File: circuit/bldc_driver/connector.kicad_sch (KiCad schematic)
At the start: 13 parts, among them J4 PH2.0_6P

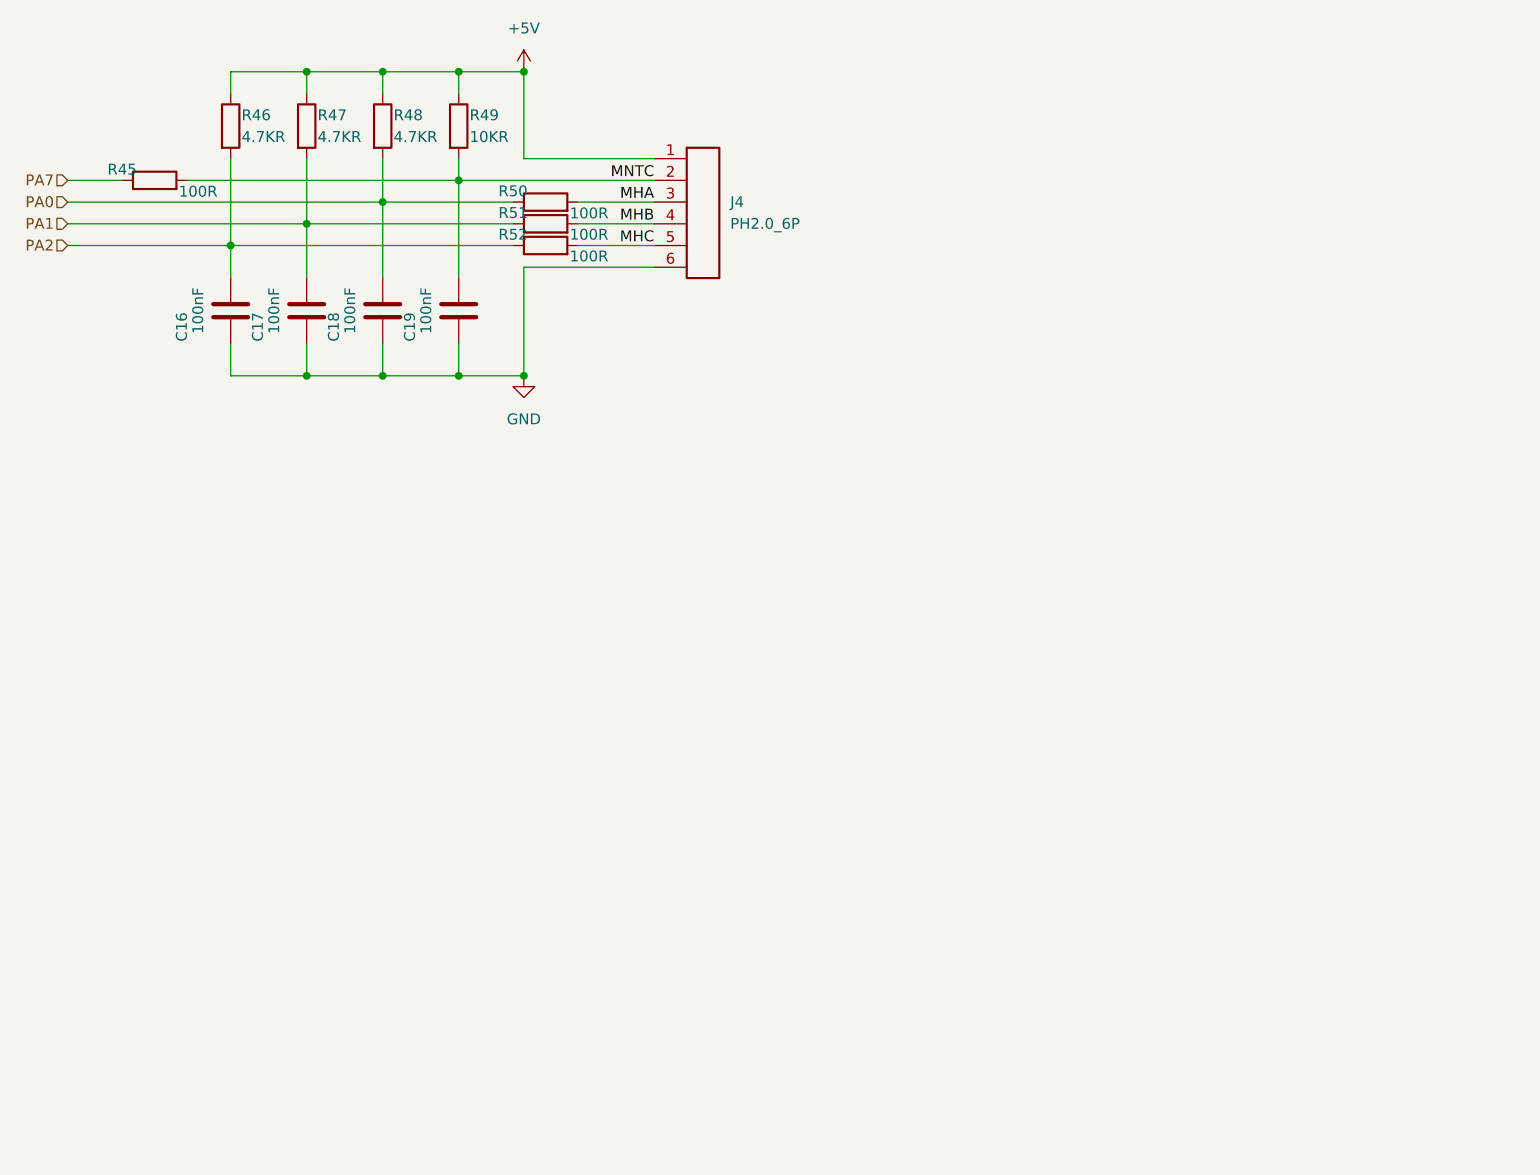
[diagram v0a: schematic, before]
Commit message: Modify the scheme of brushless motor driver board to reduce the use of resistors and capacitors to reduce the size of the circuit.
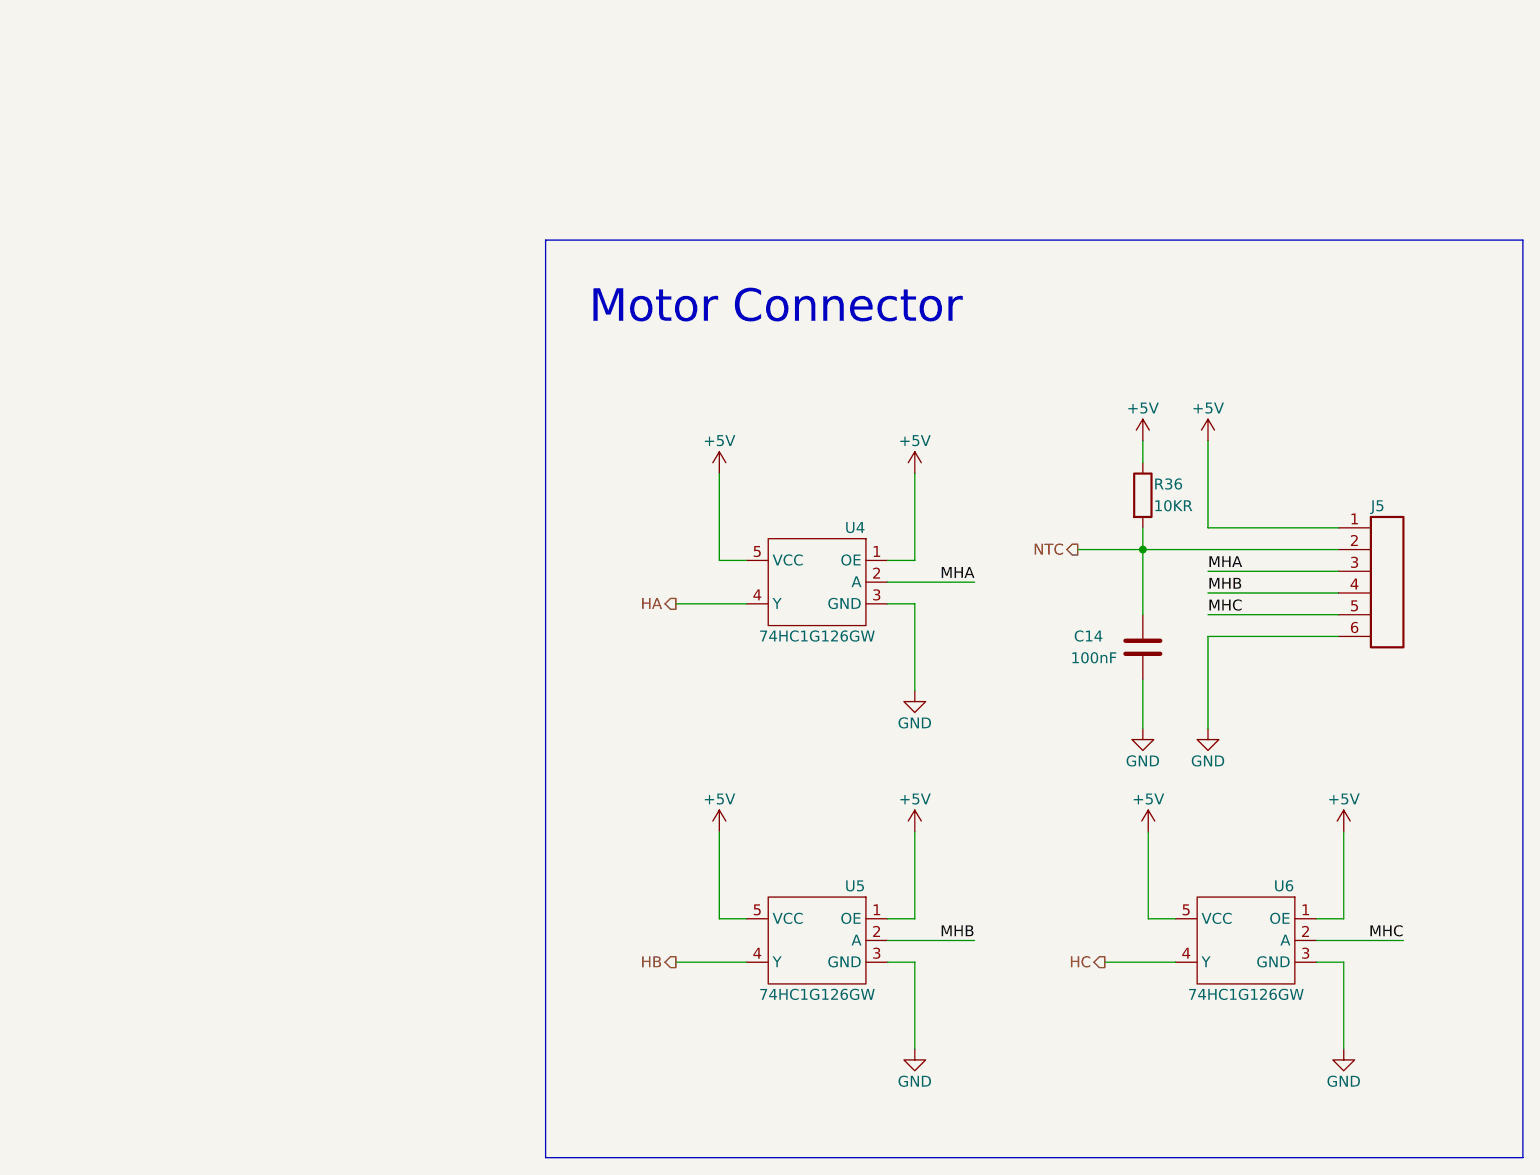
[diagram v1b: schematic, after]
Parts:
- removed C16, C17, C18: 100nF, Capacitor_SMD:C_0603_1608Metric, symbol Device:C
- removed R45, R50, R51, R52: 100R, Resistor_SMD:R_0603_1608Metric, symbol Device:R
- removed R46, R47, R48: 4.7KR, Resistor_SMD:R_0603_1608Metric, symbol Device:R
- added U4, U5, U6: 74HC1G126GW, Package_TO_SOT_SMD:SOT-353_SC-70-5, symbol Library:74HC1G126GW
- J5: renamed from J4; value PH2.0_6P -> GH1.25_6P; footprint Connector_JST:JST_PH_B6B-PH-SM4-TB_1x06-1MP_P2.00mm_Vertical -> Connector_JST:JST_GH_BM06B-GHS-TBT_1x06-1MP_P1.25mm_Vertical
- renumbered C19 to C14, R49 to R36
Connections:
- net +5V: now also U4.1 (OE), U4.5 (VCC), U5.1 (OE), U5.5 (VCC), U6.1 (OE), U6.5 (VCC)
- net GND: now also U4.3 (GND), U5.3 (GND), U6.3 (GND)
- net MHA: now also U4.2 (A)
- net MHB: now also U5.2 (A)
- net MHC: now also U6.2 (A)
- net MNTC renamed NTC
- new net HA: U4.4 (Y)
- new net HB: U5.4 (Y)
- new net HC: U6.4 (Y)
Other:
- note added: "Motor Connector"
- moved on the sheet: C14, J5, R36

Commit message: Update the schematic and package library of BLDC Driver.
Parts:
- C14: footprint Capacitor_SMD:C_0603_1608Metric -> BLDC_Driver:C_0603_1608Metric
- J5: footprint Connector_JST:JST_GH_BM06B-GHS-TBT_1x06-1MP_P1.25mm_Vertical -> BLDC_Driver:JST_GH_BM06B-GHS-TBT_1x06-1MP_P1.25mm_Vertical
- R36: footprint Resistor_SMD:R_0603_1608Metric -> BLDC_Driver:R_0603_1608Metric
- U4, U5, U6: footprint Package_TO_SOT_SMD:SOT-353_SC-70-5 -> BLDC_Driver:SOT-353_SC-70-5
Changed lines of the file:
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@@
   (title_block
     (title "BLDC Driver 6-Step")
-    (date "2022-03-25")
-    (rev "1.1.1")
+    (date "2022-03-26")
+    (rev "1.1.2")
   )
   (junction (at 160.02 85.09) (diameter 0) (color 0 0 0 0)
@@
       (effects (font (size 1.27 1.27)) (justify left) hide)
     )
-    (property "Footprint" "Connector_JST:JST_GH_BM06B-GHS-TBT_1x06-1MP_P1.25mm_Vertical" (id 2) (at 186.69 96.52 0)
+    (property "Footprint" "BLDC_Driver:JST_GH_BM06B-GHS-TBT_1x06-1MP_P1.25mm_Vertical" (id 2) (at 186.69 96.52 0)
       (effects (font (size 1.27 1.27)) hide)
     )
@@
     (property "Reference" "U5" (id 0) (at 126.365 124.46 0))
     (property "Value" "74HC1G126GW" (id 1) (at 121.92 137.16 0))
-    (property "Footprint" "Package_TO_SOT_SMD:SOT-353_SC-70-5" (id 2) (at 117.475 139.7 0)
+    (property "Footprint" "BLDC_Driver:SOT-353_SC-70-5" (id 2) (at 117.475 139.7 0)
       (effects (font (size 1.27 1.27)) hide)
     )
@@
     (property "Reference" "C14" (id 0) (at 153.67 95.25 0))
     (property "Value" "100nF" (id 1) (at 154.305 97.79 0))
-    (property "Footprint" "Capacitor_SMD:C_0603_1608Metric" (id 2) (at 159.0548 92.71 0)
+    (property "Footprint" "BLDC_Driver:C_0603_1608Metric" (id 2) (at 159.0548 92.71 0)
       (effects (font (size 1.27 1.27)) hide)
     )
@@
     (property "Reference" "U6" (id 0) (at 176.53 124.46 0))
     (property "Value" "74HC1G126GW" (id 1) (at 172.085 137.16 0))
-    (property "Footprint" "Package_TO_SOT_SMD:SOT-353_SC-70-5" (id 2) (at 167.64 139.7 0)
+    (property "Footprint" "BLDC_Driver:SOT-353_SC-70-5" (id 2) (at 167.64 139.7 0)
       (effects (font (size 1.27 1.27)) hide)
     )
@@
     (property "Reference" "U4" (id 0) (at 126.365 82.55 0))
     (property "Value" "74HC1G126GW" (id 1) (at 121.92 95.25 0))
-    (property "Footprint" "Package_TO_SOT_SMD:SOT-353_SC-70-5" (id 2) (at 117.475 97.79 0)
+    (property "Footprint" "BLDC_Driver:SOT-353_SC-70-5" (id 2) (at 117.475 97.79 0)
       (effects (font (size 1.27 1.27)) hide)
     )
@@
       (effects (font (size 1.27 1.27)) (justify left))
     )
-    (property "Footprint" "Resistor_SMD:R_0603_1608Metric" (id 2) (at 158.242 78.74 90)
-      (effects (font (size 1.27 1.27)) hide)
-    )
+    (property "Footprint" "BLDC_Driver:R_0603_1608Metric" (id 2) (at 158.242 78.74 90)
+      (effects (font (size 1.27 1.27)) hide)
+    )
